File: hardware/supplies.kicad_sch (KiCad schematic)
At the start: 19 parts, among them J11 Conn_01x02, J12 Conn_01x02, U8 AP62250WU

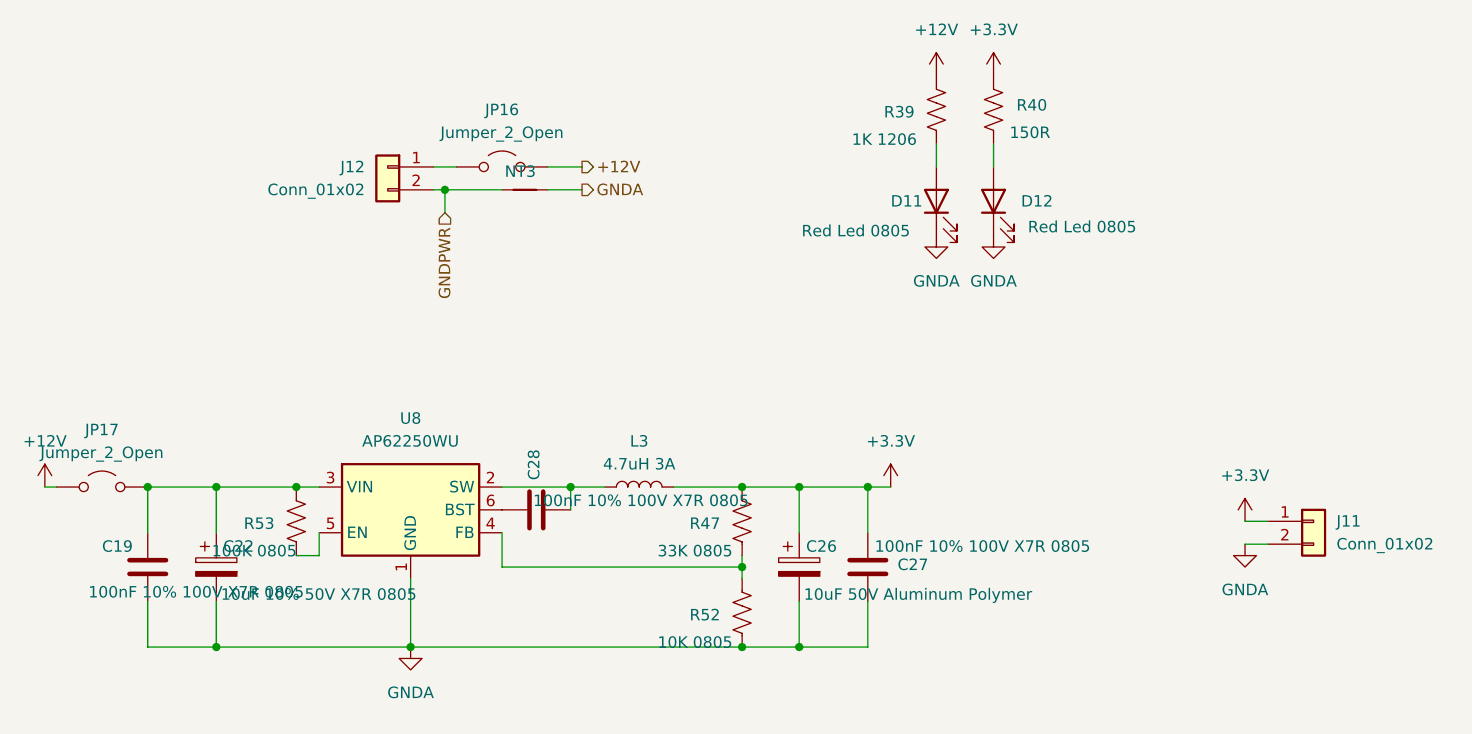
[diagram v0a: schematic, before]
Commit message: HW: PCB WIP
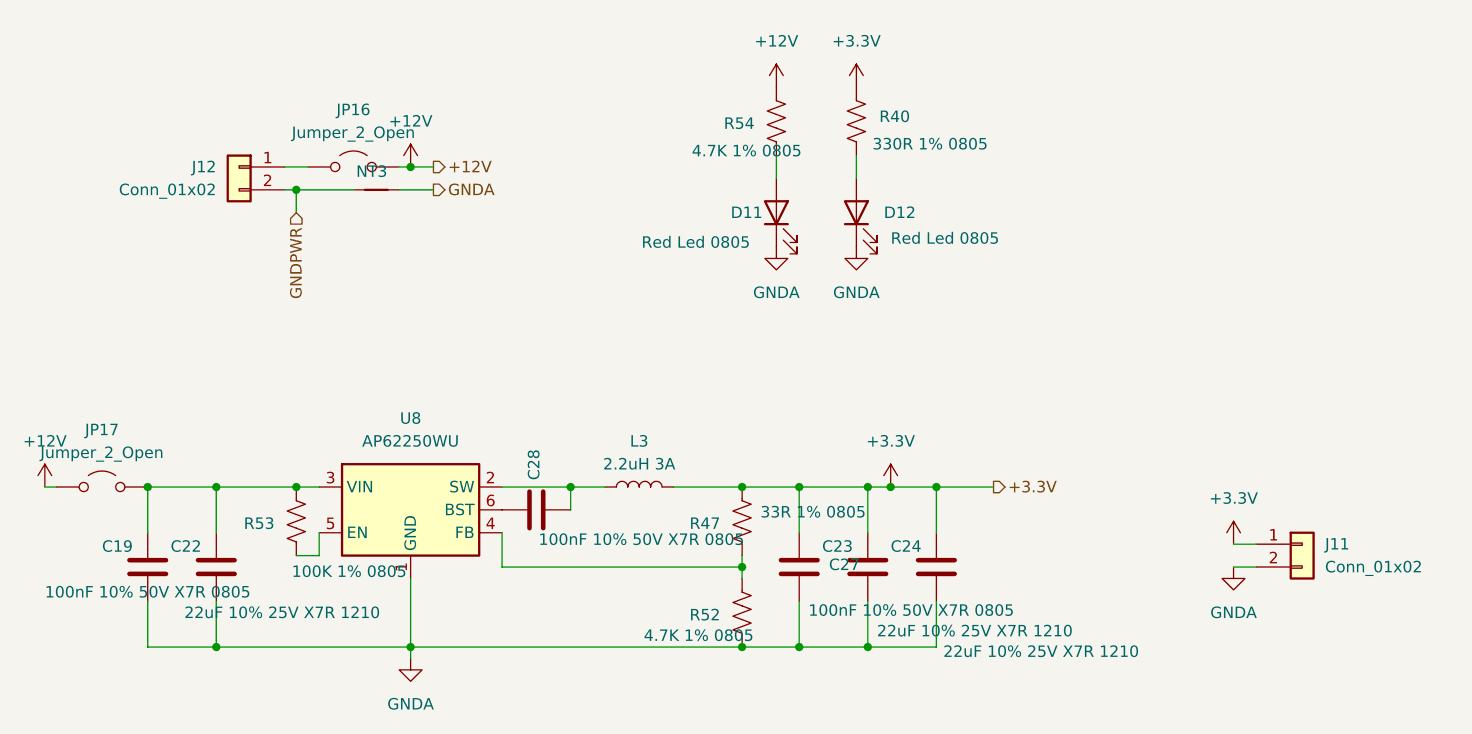
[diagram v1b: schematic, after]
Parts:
- removed C22: 10uF 10% 50V X7R 0805, Capacitor_SMD:C_0805_2012Metric_Pad1.18x1.45mm_HandSolder, symbol Device:C_Polarized
- removed C26: 10uF 50V Aluminum Polymer, Capacitor_THT:CP_Radial_D6.3mm_P2.50mm, symbol Device:C_Polarized
- removed R39: 1K 1206, Resistor_SMD:R_0805_2012Metric_Pad1.20x1.40mm_HandSolder, symbol Device:R_US
- added C22, C23, C24: 22uF 10% 25V X7R 1210, Capacitor_SMD:C_1210_3225Metric_Pad1.33x2.70mm_HandSolder, symbol Device:C
- added R54: 4.7K 1% 0805, Resistor_SMD:R_0805_2012Metric_Pad1.20x1.40mm_HandSolder, symbol Device:R_US
- C19, C27, C28: value 100nF 10% 100V X7R 0805 -> 100nF 10% 50V X7R 0805
- D11, D12: LCSC Part C19171391 -> (none)
- L3: value 4.7uH 3A -> 2.2uH 3A; footprint (none) -> Inductor_SMD_Wurth:L_Wurth_WE-LQSH-4020; LCSC Part (none) -> C122469
- R40: value 150R -> 330R 1% 0805; LCSC Part C153298 -> (none)
- R47: value 33K 0805 -> 33R 1% 0805
- R52: value 10K 0805 -> 4.7K 1% 0805; LCSC Part C153298 -> (none)
- R53: value 100K 0805 -> 100K 1% 0805
- U8: footprint Package_TO_SOT_SMD:TSOT-23-6 -> Package_TO_SOT_SMD:TSOT-23-6_HandSoldering
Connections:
- net +12V: now also R54.1
- net +3.3V: now also C23.1, C24.1
- net GNDA: now also C22.2, C23.2, C24.2
- net at D11.2 (A): now also R54.2
- net at C19.1, JP17.2 (B), R53.1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: now also C22.1
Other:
- moved on the sheet: C27, D11, D12, J11, J12, JP16, NT3, R40
